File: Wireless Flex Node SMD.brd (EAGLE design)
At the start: 81.3 x 45.6 mm, 31 parts, among them IC2 LM317, P1 2X4_HEADER, P2 2X4_HEADER

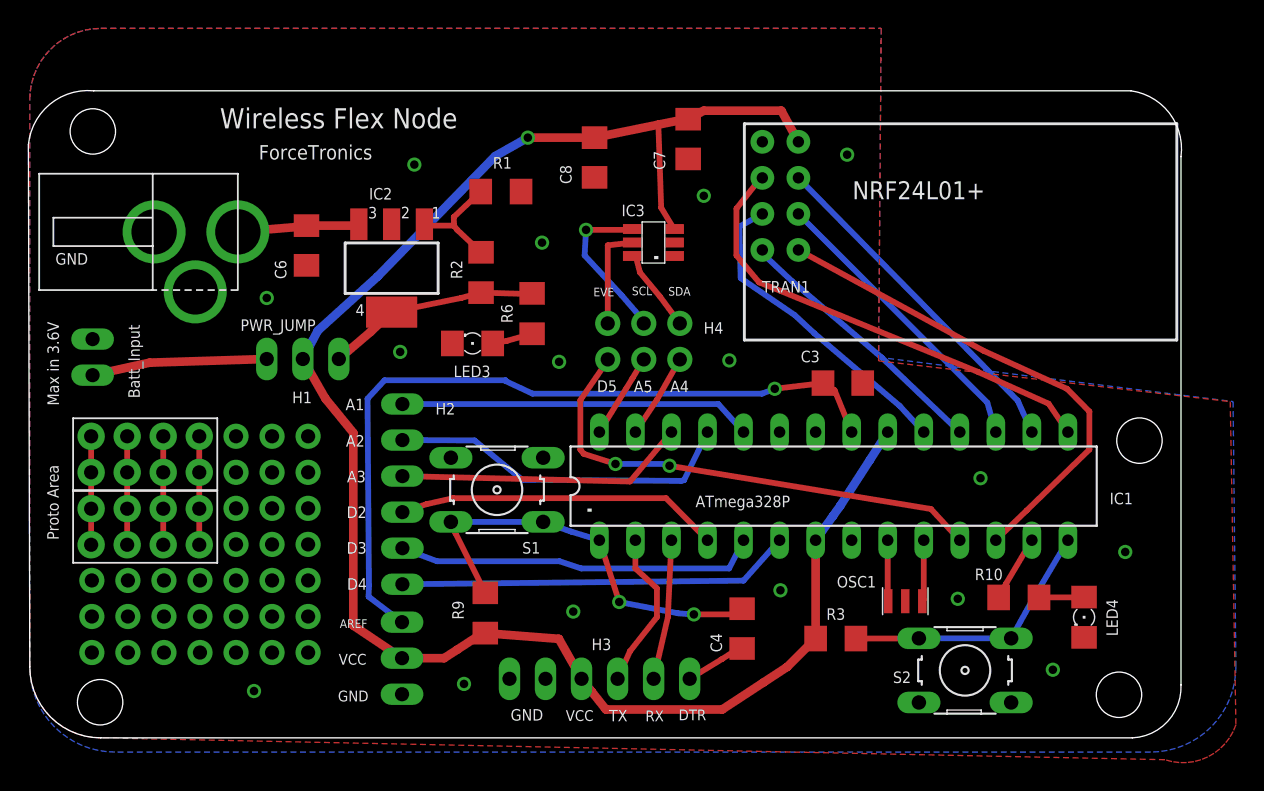
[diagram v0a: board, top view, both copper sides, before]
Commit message: Update Wireless Flex Node SMD.brd
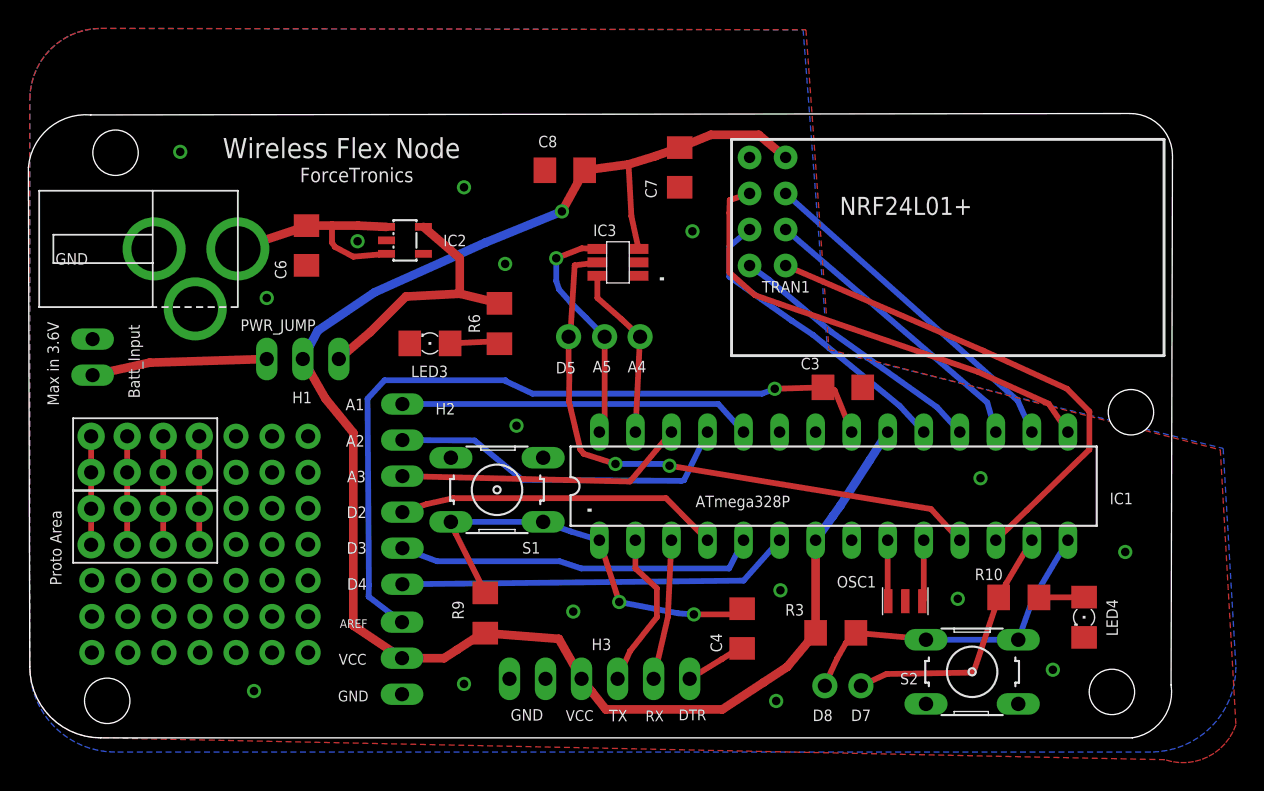
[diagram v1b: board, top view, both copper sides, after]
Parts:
- removed EVE, SCL, SDA: 2PINHEADER_S, ForceTronics:2PINHEADER_S
- removed R1: 360, rcl:R1206
- removed R2: 220, rcl:R1206
- added A4, A5, D5, D7, D8: 1PINHEADER_S, ForceTronics:1PINHEADER_S
- IC2: value LM317 -> LP2985; device linear:SOT223 -> ForceTronics:SOT23
- moved IC2 4.78 mm to (23.9, 37.6), turned to 270 degrees
- moved LED3 3.00 mm to (28.2, 27.8)
- moved U$8 2.87 mm to (42.2, 35.0)
- moved R6 2.40 mm to (33.1, 29.2)
- moved C8 2.28 mm to (37.7, 40.0), turned to 180 degrees
- moved C7 2.09 mm to (45.8, 40.2)
- moved NRF24L01+ 1.42 mm to (49.5, 26.9)
- moved N3 1.20 mm to (0.66, 38.6)
- moved S2 0.51 mm to (66.4, 4.65)
- moved R3 0.40 mm to (56.8, 7.40)
- moved C3 0.30 mm to (57.3, 24.7)
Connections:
- removed net N$27: DGHDFGH.28, SCL.N1
- removed net N$29: DGHDFGH.27, SDA.N1
- removed net N$30: EVE.N0, U$8.5
- removed net N$31: DGHDFGH.11, EVE.N1
- removed net N$33: IC2.1, R1.2, R2.1
- new net A5: D5.P$1, DGHDFGH.11, U$8.5
- net GND: now also IC2.2; no longer R1.1
- net N$11: now also D7.P$1
- net N$16: now also D8.P$1
- net N$26: now also A5.P$1, DGHDFGH.28; no longer SCL.N0
- net N$28: now also A4.P$1, DGHDFGH.27; no longer SDA.N0
- net N$32: now also IC2.1
- net N$34: now also IC2.5; no longer IC2.4, R2.2
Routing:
- net A5: track 0.00 -> 43.1 mm, vias 0 -> 2
- net N$31: track 35.3 -> 0.00 mm, vias 2 -> 0
- net N$11: track 4.66 -> 18.4 mm
- net N$33: track 8.08 -> 0.00 mm
- net N$32: track 8.68 -> 16.2 mm
- net N$30: track 7.28 -> 0.00 mm
- net N$28: track 5.96 -> 12.4 mm
- net N$29: track 6.00 -> 0.00 mm
- net N$27: track 6.00 -> 0.00 mm
- net N$26: track 11.5 -> 17.0 mm
- net N$16: track 18.9 -> 23.8 mm
- net VCC: track 125.1 -> 121.0 mm
- net N$34: track 15.0 -> 19.0 mm
- net N$36: track 2.86 -> 4.56 mm
- net N$3: track 22.4 -> 21.6 mm
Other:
- board size 81.3 x 45.6 mm -> 80.6 x 44 mm
- board text added: "D7"
- board text added: "D8"
- board text added: "ForceTronics.com"
- board text removed: "H4"
